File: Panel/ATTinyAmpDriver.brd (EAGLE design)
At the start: 51 x 51 mm, 125 parts, among them Q1 SI2301CDS, Q2 BC846, Q3 SI2301CDS, Q4 BC846, Q5 SI2301CDS, Q6 BC846, Q7 SI2301CDS, Q8 BC846, U1 SPX5205M5-L-3-3, U10 SPX5205M5-L-3-3, U11 ATTINY5-TSHR, U12 MCP6L2-X_SN, U2 ATTINY5-TSHR, U3 MCP6L2-X_SN, U4 SPX5205M5-L-3-3, U5 ATTINY5-TSHR, U6 MCP6L2-X_SN, U7 SPX5205M5-L-3-3, U8 ATTINY5-TSHR, U9 MCP6L2-X_SN, X1 DIODES, X2 INPUT, X3 INPUT, X4 DIODES, X5 INPUT, X6 DIODES, X7 INPUT, X8 DIODES

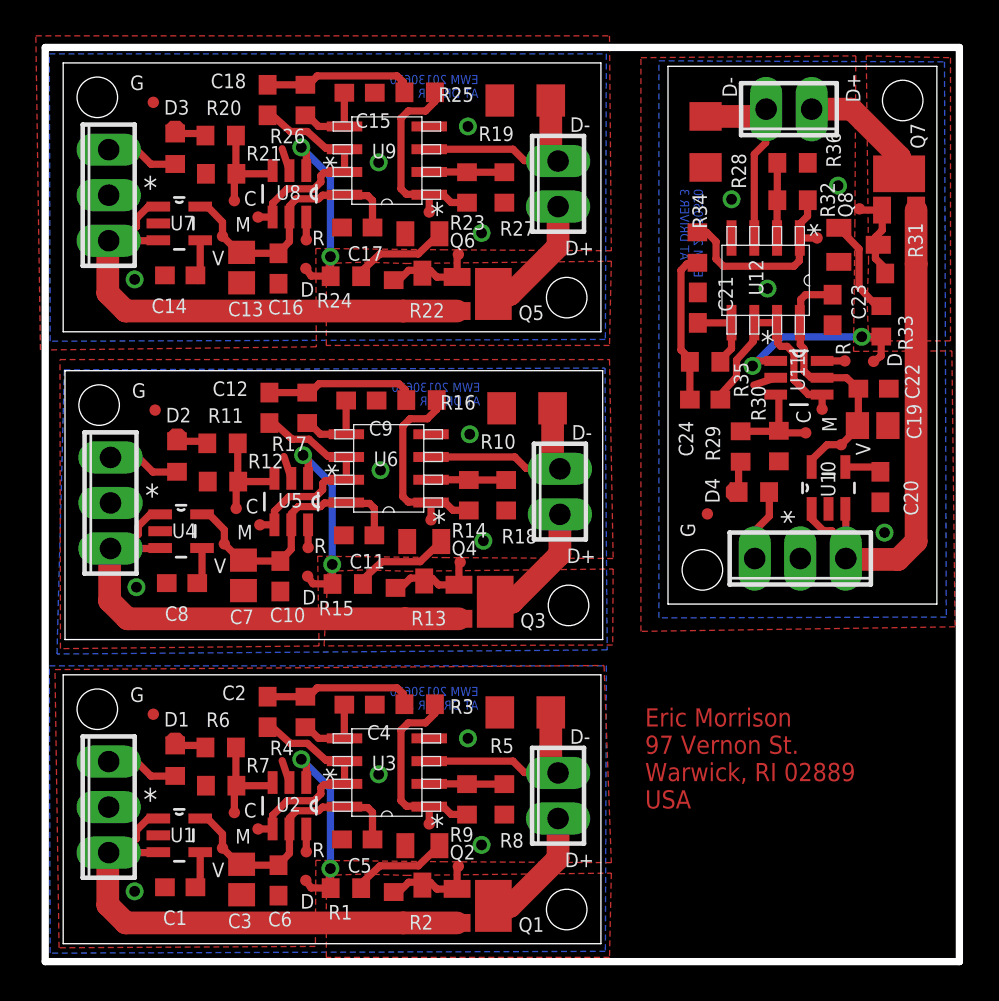
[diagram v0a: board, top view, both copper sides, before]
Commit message: Panel Change
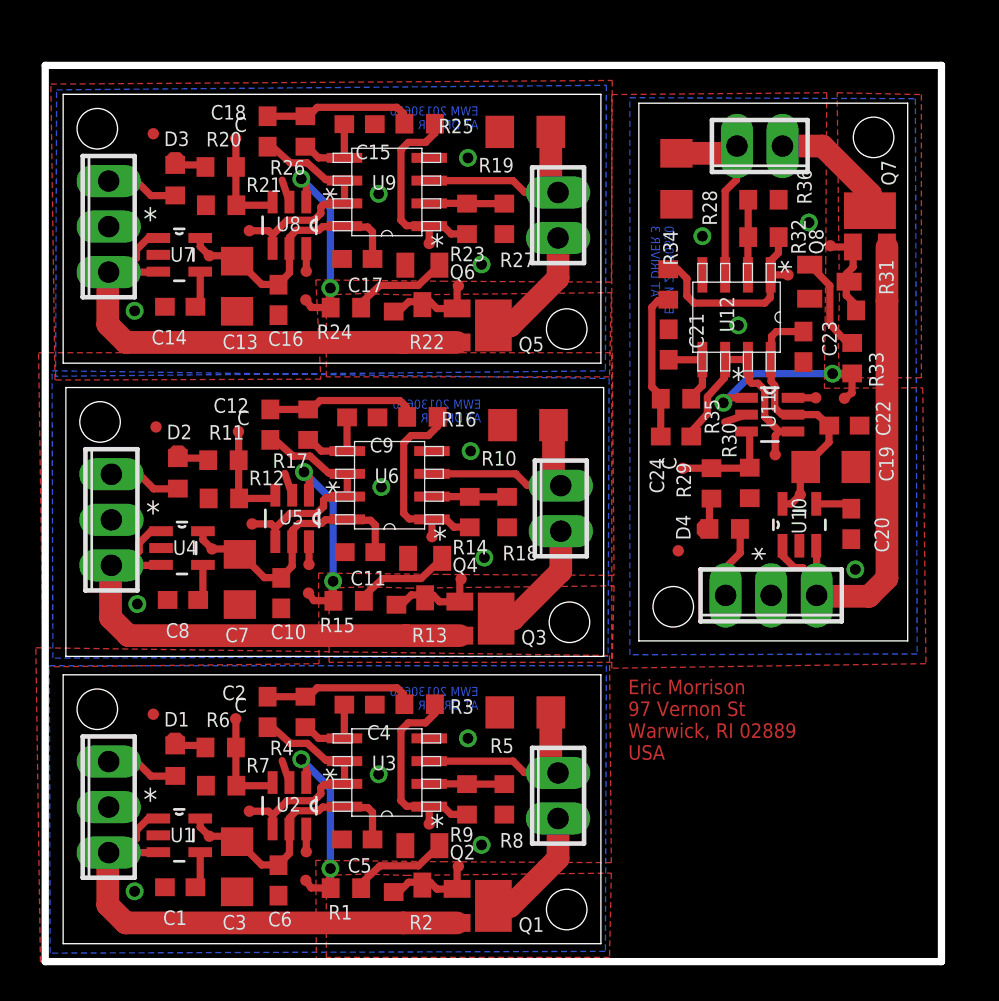
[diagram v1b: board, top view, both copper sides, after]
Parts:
- C13, C19, C3, C7: value 10u -> 47u; device resistor:C0805 -> resistor:C1206
- moved TPICLK3 7.14 mm to (34.6, 26.5)
- moved TPICLK 5.23 mm to (9.63, 12.5)
- moved TPICLK1 4.29 mm to (9.78, 28.6)
- moved MEASURE3 3.65 mm to (39.7, 27.3)
- moved +5V3 3.61 mm to (41.1, 25.0)
- moved TPICLK2 3.48 mm to (9.63, 44.9)
- moved C19 3.29 mm to (42.8, 26.6)
- moved C21 2.62 mm to (33.8, 33.4)
- moved R30 2.62 mm to (38.3, 25.7)
- moved R32 2.62 mm to (39.1, 39.4)
- moved R36 2.62 mm to (39.1, 41.5)
- moved RESET3 2.62 mm to (42.0, 30.5)
- moved TPIDATA3 2.62 mm to (43.6, 30.4)
- moved C20 2.62 mm to (44.0, 23.4)
- moved C22 2.62 mm to (43.6, 28.9)
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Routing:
- net MEASURE1: track 12.8 -> 13.4 mm
- net MEASURE: track 12.8 -> 13.4 mm
- net MEASURE3: track 12.8 -> 13.4 mm
- net MEASURE2: track 12.8 -> 13.4 mm
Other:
- board size 51 x 51 mm -> 50 x 50 mm
- board text added: "Eric Morrison 97 Vernon St Warwick, RI 02889 USA"
- board text removed: "01-16"
- board text removed: "01-20"
- board text removed: "Eric Morrison 97 Vernon St. Warwick, RI 02889 USA"
- board text removed: "LAYER-STACK"
